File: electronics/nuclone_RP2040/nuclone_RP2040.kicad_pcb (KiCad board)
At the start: 4 copper layers, 50 x 50 mm, 64 parts, among them J1 JTAG_2X05, J2 TYPE-C-31-M-12, J3 nuclone_small_left, J4 nuclone_small_right, J5 Conn_02x06_Odd_Even, SW1 RESET, SW2 Bootloader, U1 MCP1702-MB, U2 TPESD0504C6, U3 rp2040, U4 MX25L3233FZBI, Y1 12MHz

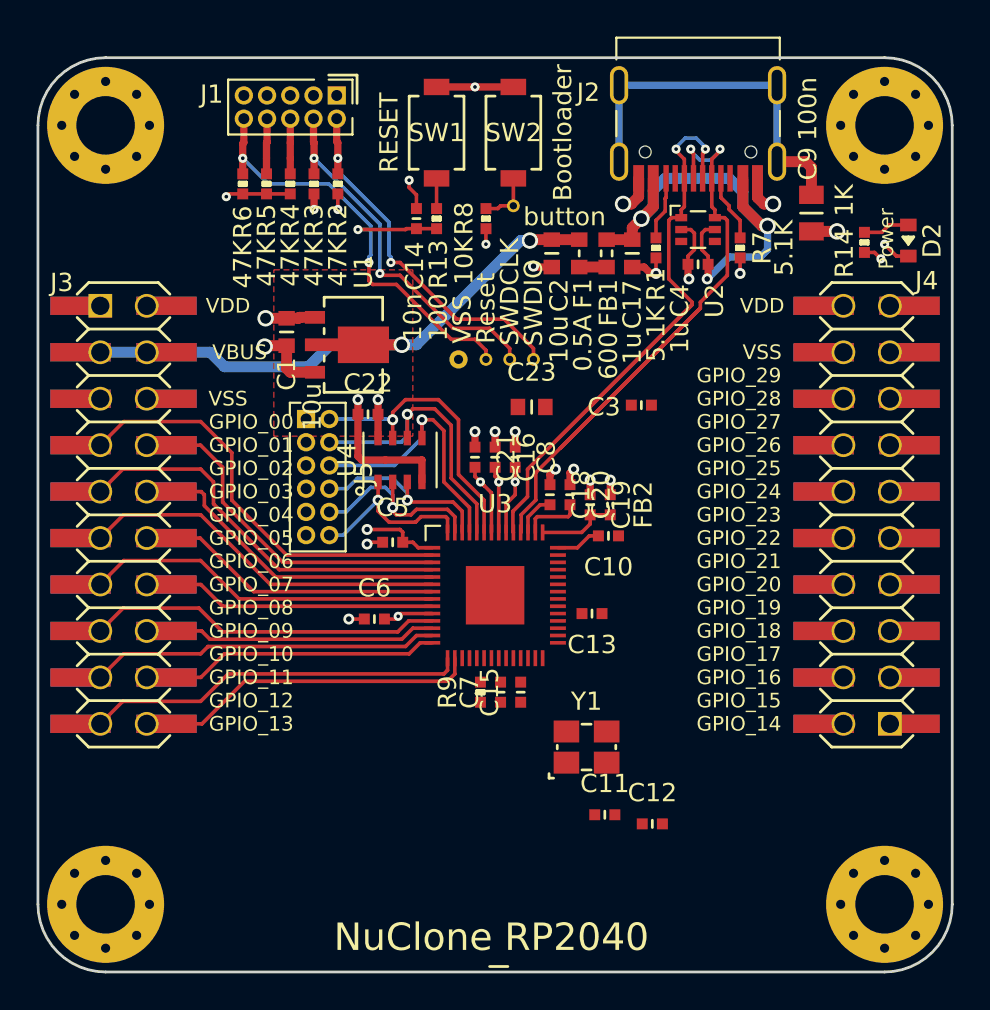
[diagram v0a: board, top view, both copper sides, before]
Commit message: further routing in progress
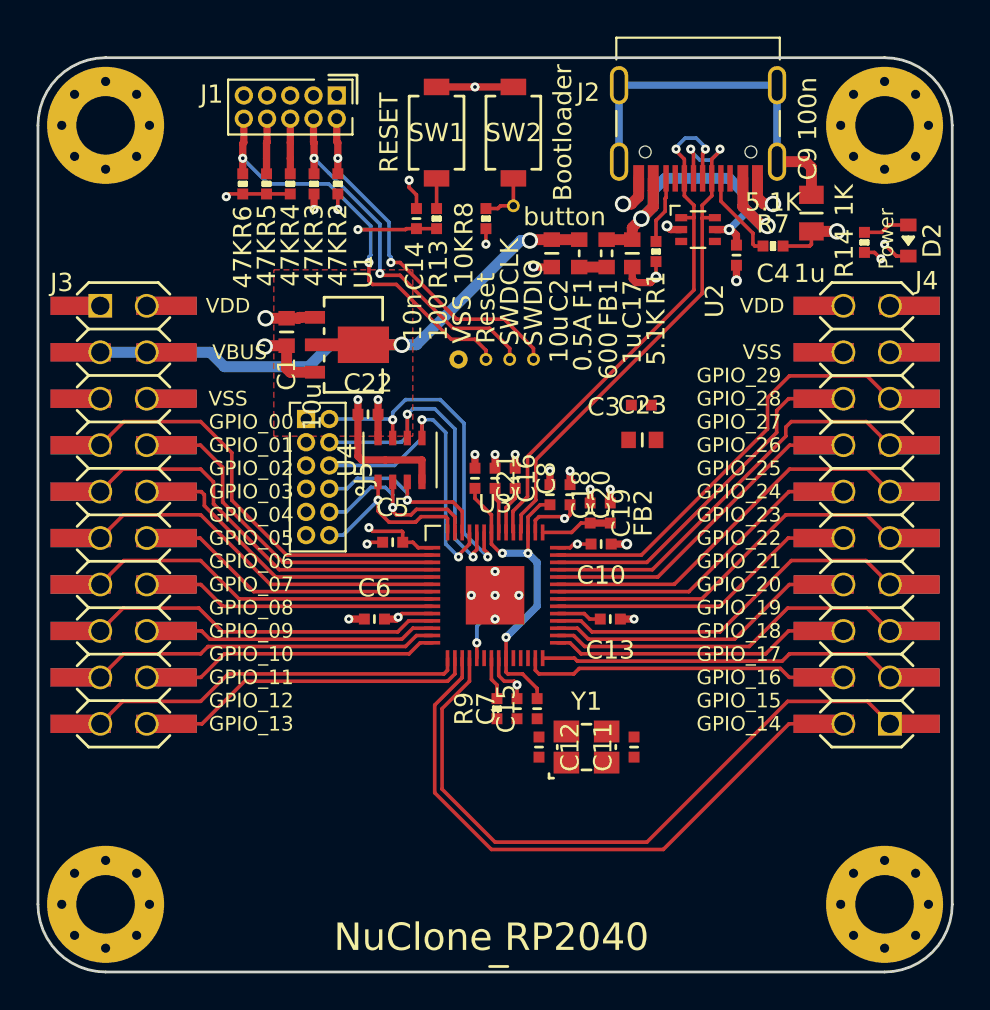
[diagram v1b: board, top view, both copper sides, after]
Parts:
- moved C12 7.49 mm to (87.4, 98.7), turned to -90 degrees
- moved C23 6.31 mm to (93.0, 81.9)
- moved C11 4.03 mm to (92.6, 98.7), turned to 90 degrees
- moved C4 2.16 mm to (98.2, 71.8), turned to -90 degrees
- moved R7 1.80 mm to (100.2, 71.3), turned to 180 degrees
- moved C7 1.27 mm to (86.2, 96.6)
- moved C15 1.27 mm to (87.3, 96.6)
- moved R9 1.27 mm to (85.1, 96.6)
- moved C16 1.15 mm to (85.0, 84.0)
- moved C21 1.15 mm to (83.9, 84.0)
- moved C8 1.15 mm to (86.1, 84.0)
- moved C13 1.04 mm to (91.3, 91.7)
- moved C10 0.60 mm to (90.8, 87.6)
- moved C19 0.45 mm to (90.2, 85.9)
- moved FB2 0.45 mm to (91.3, 85.9)
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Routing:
- net /GPIO_15: track 0.00 -> 37.2 mm
- net /GPIO_14: track 0.00 -> 33.4 mm
- net /GPIO_29: track 0.00 -> 23.7 mm
- net /GPIO_27: track 0.00 -> 22.3 mm
- net /GPIO_25: track 0.00 -> 21.3 mm
- net /GPIO_23: track 0.00 -> 20.6 mm
- net /GPIO_21: track 0.00 -> 20.6 mm
- net /GPIO_19: track 0.00 -> 19.8 mm
- net /GPIO_17: track 0.00 -> 19.8 mm
- net /GPIO_28: track 0.00 -> 18.9 mm
- net /GPIO_26: track 0.00 -> 17.5 mm
- net /GPIO_16: track 0.00 -> 16.8 mm
- net /GPIO_24: track 0.00 -> 16.8 mm
- net /GPIO_22: track 0.00 -> 16.1 mm
- net /GPIO_20: track 0.00 -> 16.0 mm
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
